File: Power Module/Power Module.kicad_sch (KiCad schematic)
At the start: 21 parts, among them J6 Conn_02x12_Odd_Even, U1 LM2576S-3.3

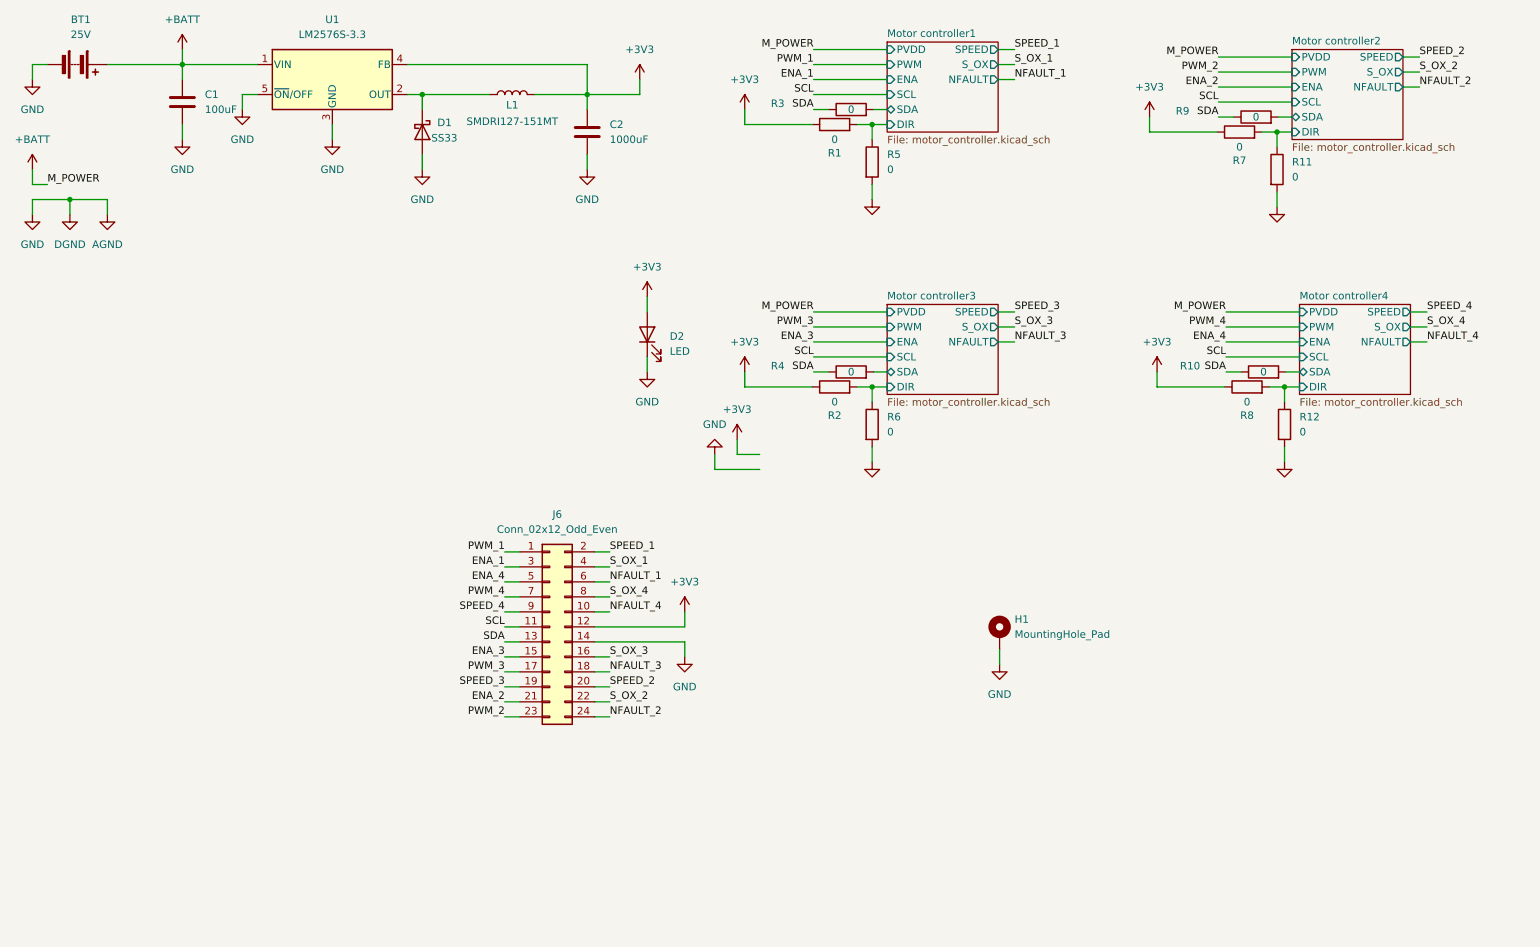
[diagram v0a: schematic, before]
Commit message: V1 design
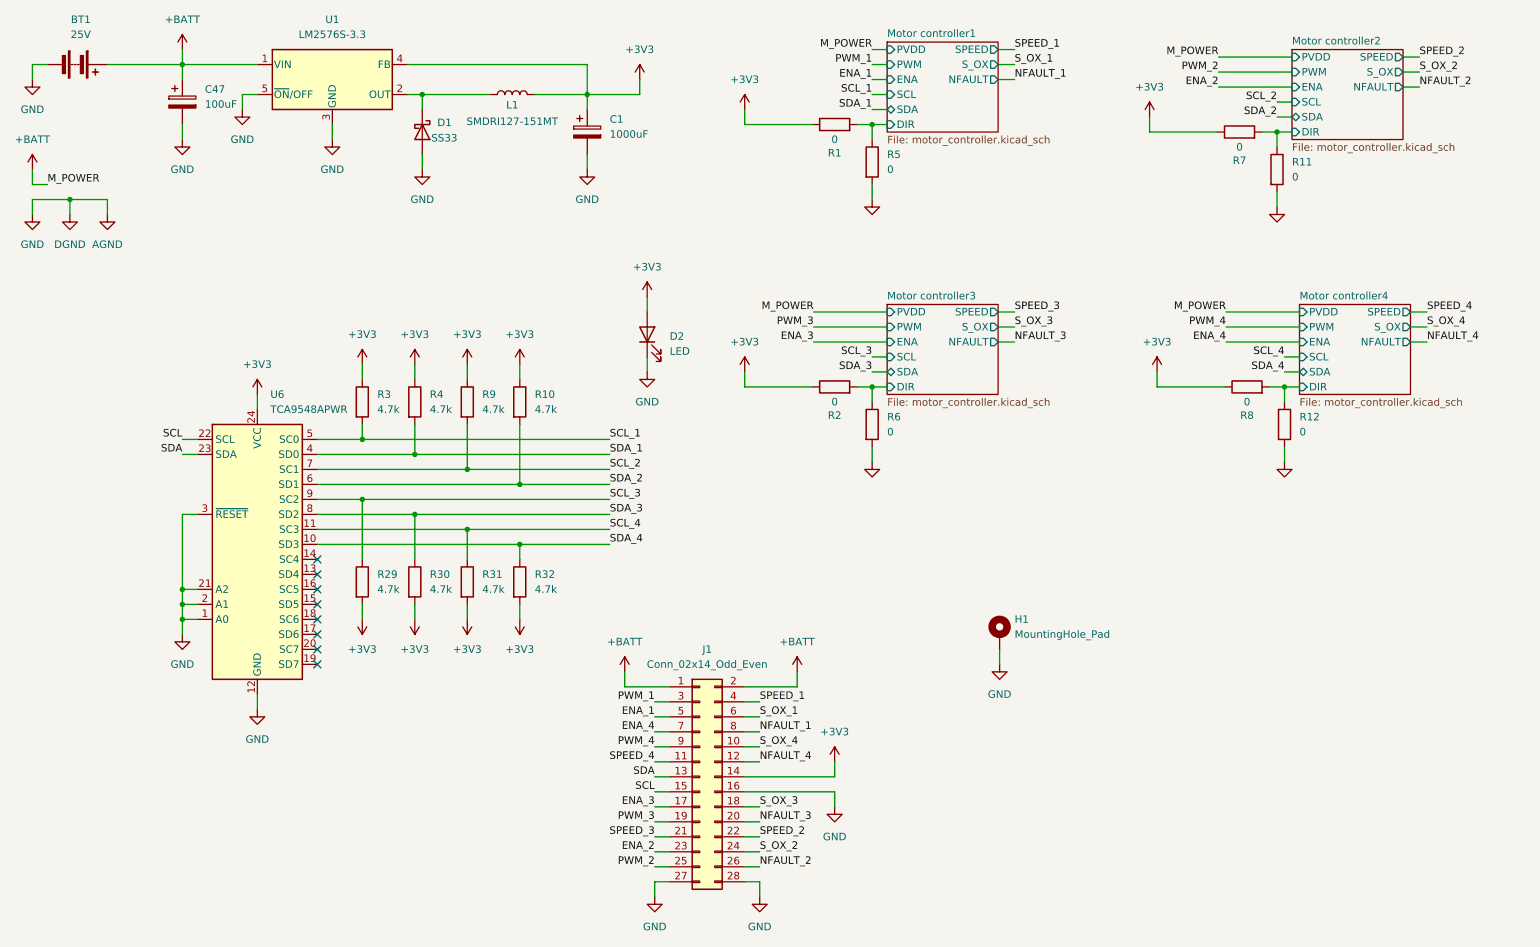
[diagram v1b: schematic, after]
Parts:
- removed C1: 100uF, Capacitor_SMD:C_0603_1608Metric, symbol Device:C
- removed C2: 1000uF, Capacitor_SMD:C_0603_1608Metric, symbol Device:C
- removed J6: Conn_02x12_Odd_Even, Connector_PinHeader_2.54mm:PinHeader_2x12_P2.54mm_Vertical, symbol Connector_Generic:Conn_02x12_Odd_Even
- added C1: 1000uF, Capacitor_Tantalum_SMD:CP_EIA-7343-30_AVX-N, symbol Device:C_Polarized
- added C47: 100uF, Capacitor_Tantalum_SMD:CP_EIA-7343-43_Kemet-X, symbol Device:C_Polarized
- added J1: Conn_02x14_Odd_Even, Connector_PinHeader_2.54mm:PinHeader_2x14_P2.54mm_Vertical, symbol Connector_Generic:Conn_02x14_Odd_Even
- added R29, R30, R31, R32: 4.7k, Resistor_SMD:R_0402_1005Metric, symbol Device:R
- added U6: TCA9548APWR, Package_SO:TSSOP-24_4.4x7.8mm_P0.65mm, symbol Interface_Expansion:TCA9548APWR
- R10, R3, R4, R9: value 0 -> 4.7k; footprint Resistor_SMD:R_0603_1608Metric_Pad0.98x0.95mm_HandSolder -> Resistor_SMD:R_0402_1005Metric
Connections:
- net +3V3: now also R10.1, R3.1, R4.1, R9.1, C1.1, J1.14 (Pin_14), R29.2, R30.2, R31.2, R32.2, U6.24 (VCC)
- net +BATT: now also C47.1, J1.1 (Pin_1), J1.2 (Pin_2)
- net AGND: now also C1.2, C47.2, J1.16 (Pin_16), J1.27 (Pin_27), J1.28 (Pin_28), U6.1 (A0), U6.12 (GND), U6.2 (A1), U6.21 (A2), U6.3 (~{RESET})
- net ENA_1: now also J1.5 (Pin_5)
- net ENA_2: now also J1.23 (Pin_23)
- net ENA_3: now also J1.17 (Pin_17)
- net ENA_4: now also J1.7 (Pin_7)
- net NFAULT_1: now also J1.8 (Pin_8)
- net NFAULT_2: now also J1.26 (Pin_26)
- net NFAULT_3: now also J1.20 (Pin_20)
- net NFAULT_4: now also J1.12 (Pin_12)
- net PWM_1: now also J1.3 (Pin_3)
- net PWM_2: now also J1.25 (Pin_25)
- net PWM_3: now also J1.19 (Pin_19)
- net PWM_4: now also J1.9 (Pin_9)
- net SCL: now also J1.15 (Pin_15), U6.22 (SCL)
- net SDA: now also J1.13 (Pin_13), U6.23 (SDA); no longer R10.1, R3.1, R4.1, R9.1
- net SPEED_1: now also J1.4 (Pin_4)
- net SPEED_2: now also J1.22 (Pin_22)
- net SPEED_3: now also J1.21 (Pin_21)
- net SPEED_4: now also J1.11 (Pin_11)
- net S_OX_1: now also J1.6 (Pin_6)
- net S_OX_2: now also J1.24 (Pin_24)
- net S_OX_3: now also J1.18 (Pin_18)
- net S_OX_4: now also J1.10 (Pin_10)
- net Motor controller1/SDA renamed SCL_1
- net SCL_1: now also U6.5 (SC0)
- net Motor controller2/SDA renamed SCL_2
- net SCL_2: now also U6.7 (SC1)
- net Motor controller3/SDA renamed SDA_1
- net SDA_1: now also U6.4 (SD0)
- net Motor controller4/SDA renamed SDA_2
- net SDA_2: now also U6.6 (SD1)
- new net SCL_3: R29.1, U6.9 (SC2)
- new net SCL_4: R31.1, U6.11 (SC3)
- new net SDA_3: R30.1, U6.8 (SD2)
- new net SDA_4: R32.1, U6.10 (SD3)
- no-connect marks 0 -> 8
